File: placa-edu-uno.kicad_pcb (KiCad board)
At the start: 2 copper layers, 97.1 x 58.9 mm, 56 parts, among them J1 Conn_02x20_Odd_Even_MountingP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, J10 HEADER, J11 HEADER, J12 HEADER, J13 HEADER, J14 HEADER, J15 HEADER, J3 Screw_Terminal_01x02, J4 Screw_Terminal_01x02, J5 Screw_Terminal_01x02, J6 Conn_02x13_Odd_Even, J7 HEADER, J8 HEADER, J9 HEADER, U1 PCA9685PW_118, U2 MAX98357AETE_T, U3 MAX98357AETE_T, U4 ICS-43434, U5 ICS-43434

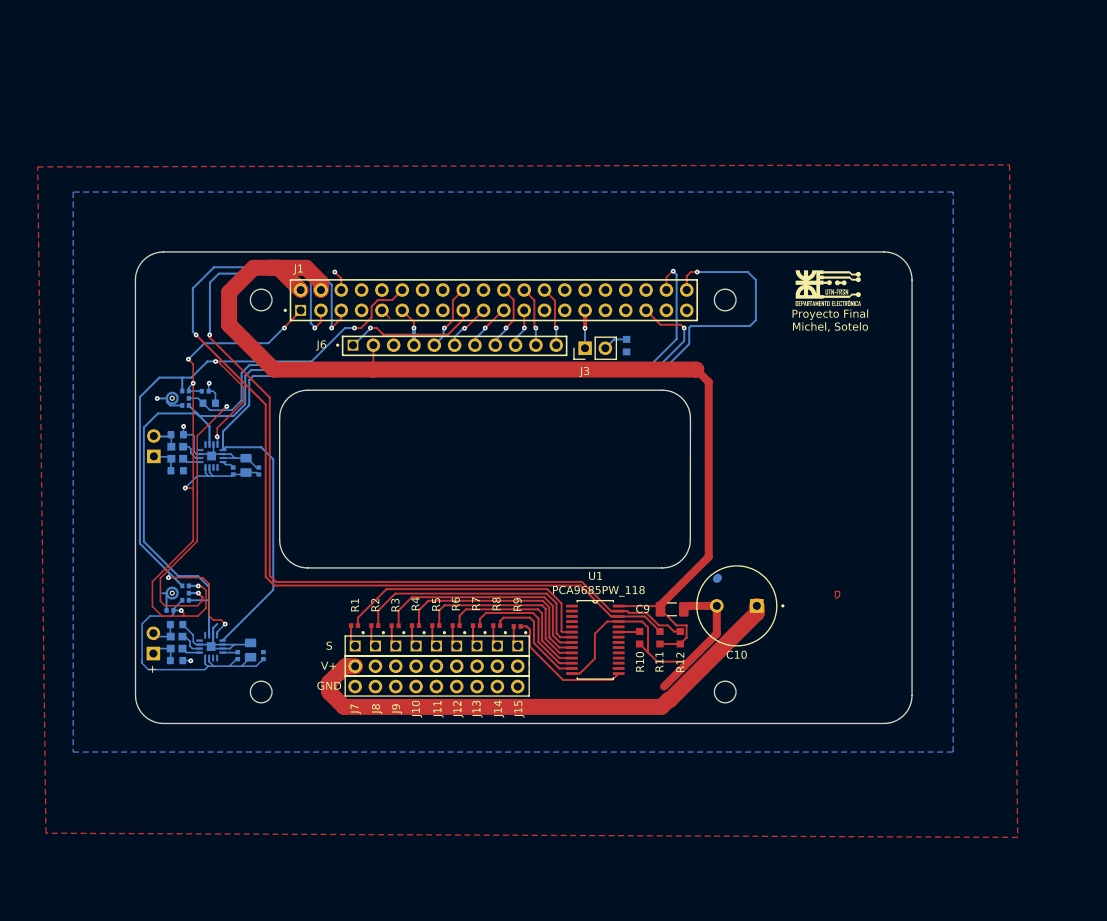
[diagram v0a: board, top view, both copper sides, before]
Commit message: Se borro todo y se arranco de nuevo. Placa circular.
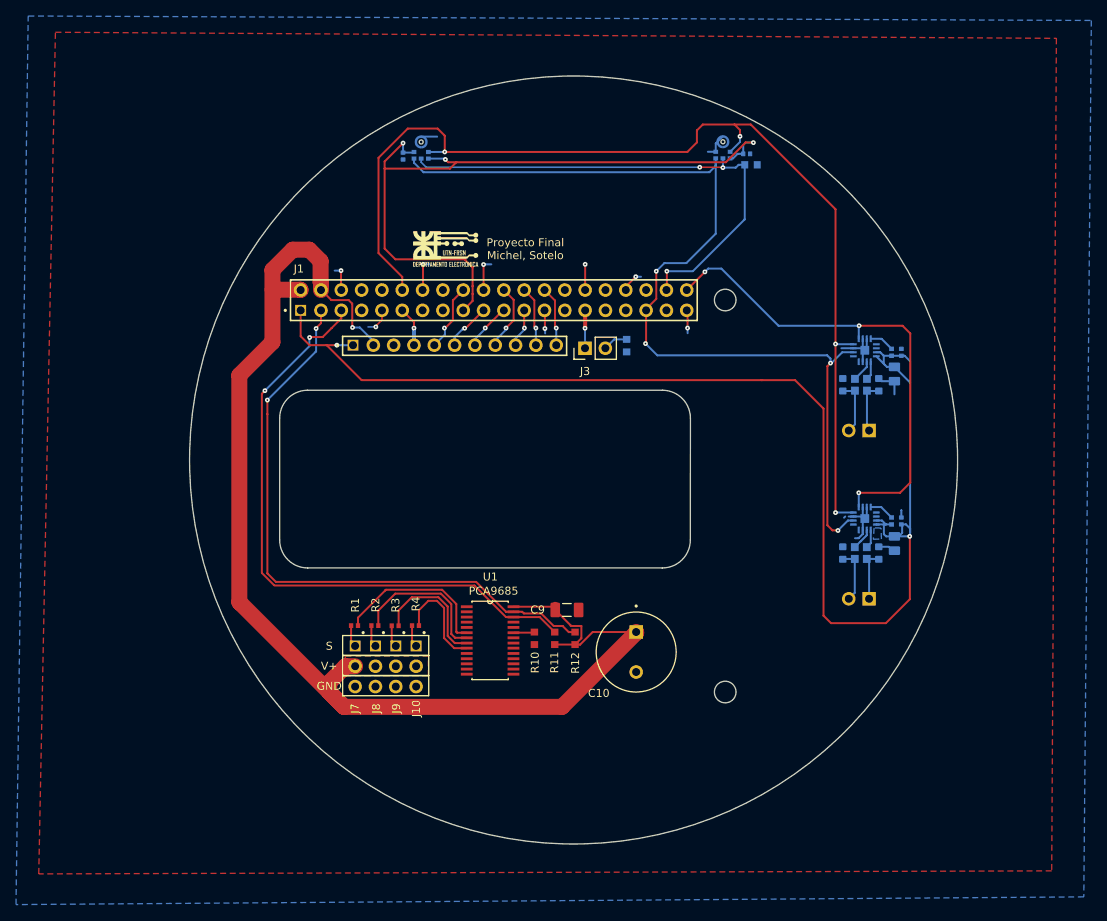
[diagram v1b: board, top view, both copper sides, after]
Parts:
- removed J11, J12, J13, J14, J15: HEADER, TSW-101-07-T-T:SAMTEC_TSW-101-07-T-T
- removed the MountingHole at (3.50, 3.50)
- removed the MountingHole at (3.50, 52.5)
- removed R5, R6, R7, R8, R9: 220, RC0402FR-07220RL:RESC1005X40N
- U1: value PCA9685PW_118 -> PCA9685
- U2, U3: value MAX98357AETE_T -> MAX98357A
- moved C8 88.8 mm to (80.7, 35.1), turned to 90 degrees
- moved C4 88.3 mm to (80.7, 14.1), turned to -90 degrees
- moved FL3 87.1 mm to (79.2, 35.1), turned to -90 degrees
- moved FL1 86.7 mm to (79.2, 14.1), turned to -90 degrees
- moved FL4 85.4 mm to (77.7, 35.1), turned to -90 degrees
- moved FL2 85.1 mm to (77.7, 14.1), turned to -90 degrees
- moved C7 83.8 mm to (76.2, 35.1), turned to 90 degrees
- moved R13 83.6 mm to (82.3, 10.0)
- moved J5 83.6 mm to (73.6, 40.9), turned to 90 degrees
- moved J4 83.6 mm to (73.6, 19.8), turned to 90 degrees
- moved R14 83.4 mm to (82.3, 31.1)
- moved C3 83.4 mm to (76.2, 14.1), turned to 90 degrees
- moved U3 83.3 mm to (78.9, 30.8), turned to -90 degrees
- moved U2 82.7 mm to (78.9, 9.78), turned to -90 degrees
- moved C2 81.9 mm to (82.7, 12.7), turned to -90 degrees
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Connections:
- C10 pad 1: 5V_Fuente -> 5V_RPI
- J10 pad 02: 5V_Fuente -> 5V_RPI
- J7 pad 02: 5V_Fuente -> 5V_RPI
- J8 pad 02: 5V_Fuente -> 5V_RPI
- J9 pad 02: 5V_Fuente -> 5V_RPI
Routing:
- net 3.3V_RPI: track 130.1 -> 257.8 mm, vias 7 -> 5
- net 5V_Fuente: track 65.2 -> 0.00 mm
- net GPIO_21_DOUT_PCM: track 126.1 -> 61.5 mm, vias 1 -> 3
- net GPIO_20_DIN_PCM: track 115.5 -> 64.2 mm
- net GPIO_3_SCL_I2C: track 119.4 -> 77.5 mm
- net GPIO_18_CLK_PCM: track 94.3 -> 134.5 mm, vias 5 -> 4
- net GPIO_2_SDA_I2C: track 116.3 -> 77.7 mm
- net GND: track 89.8 -> 54.6 mm, vias 5 -> 8
- net 5V_RPI: track 135.1 -> 159.9 mm, vias 0 -> 1
- net /Driver Servos/J4: track 23.4 -> 0.00 mm
- net /Driver Servos/J5: track 20.1 -> 0.00 mm
- net /Driver Servos/J6: track 17.0 -> 0.00 mm
- net /Driver Servos/J8: track 16.6 -> 0.00 mm
- net /Driver Servos/J7: track 13.9 -> 0.00 mm
- net /Driver Servos/J0: track 33.5 -> 20.3 mm
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- added copper zone on F.Cu, net 5V_RPI
- removed copper zone on F.Cu, net 5V_Fuente
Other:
- board size 97.1 x 58.9 mm -> 96 x 96 mm
